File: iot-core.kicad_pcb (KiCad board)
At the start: 2 copper layers, 34 x 61.2 mm, 49 parts, among them P1 USB, P10 CONN_01X01, P11 CONN_01X01, P2 CONN_01X02, P3 CONN_01X16, P4 CONN_01X04, P5 CONN_01X16, P6 CONN_01X03, P7 CONN_01X03, P8 CONN_01X01, P9 CONN_01X01, SW1 SW1, SW2 SW_PUSH_SMALL_H, U1 LP2985LV, U2 STM32F103C8Tx, U3 ESP-07v2, Y1 8MHz

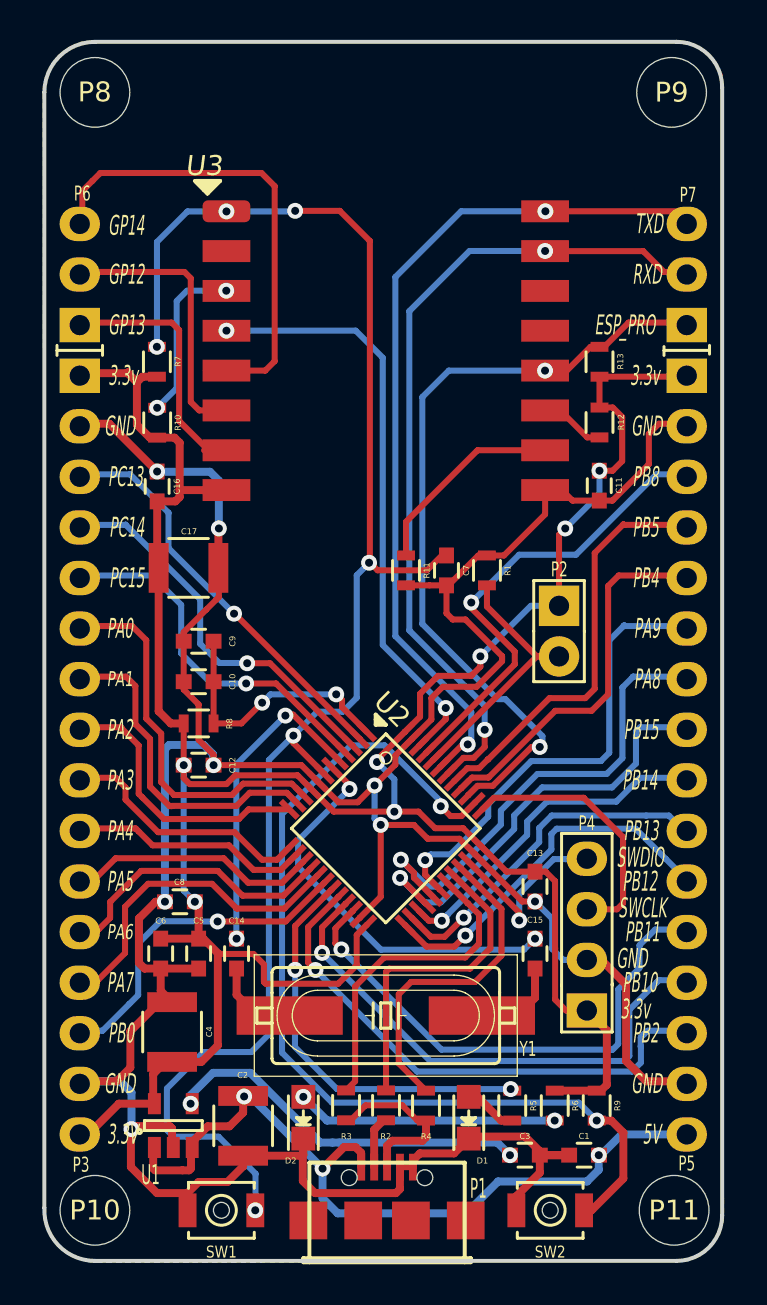
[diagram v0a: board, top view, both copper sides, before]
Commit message: Modified README file, rename project, add gerber file, anh 3d. ADD lib ESP8266 & BUTTON
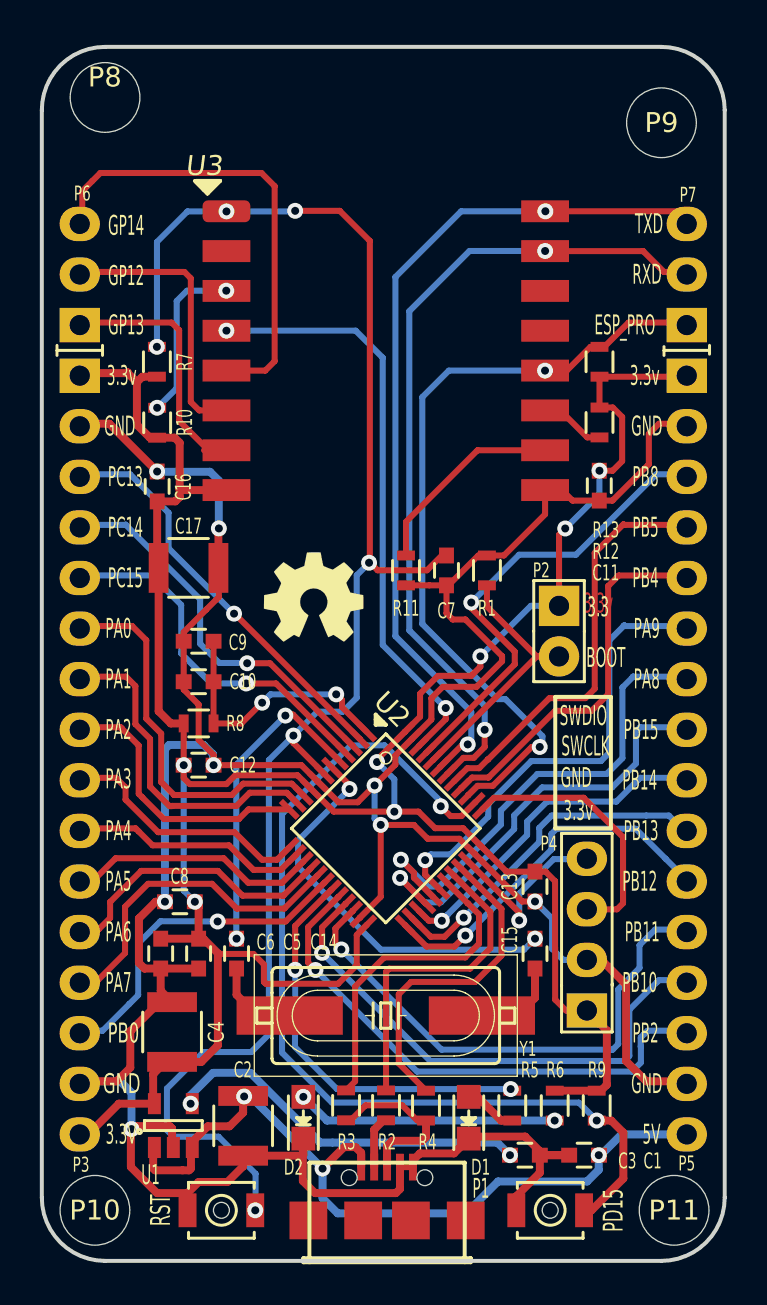
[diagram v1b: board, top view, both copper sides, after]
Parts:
- added G***: logo5_silkscreen-front_5mm, logo:logo5_silkscreen-front_5mm, F.Cu at (118.4, 102.6)
- SW1: value SW1 -> RST
- moved P9 1.61 mm to (135.9, 78.7)
- moved P8 0.57 mm to (108.0, 77.5)
- renumbered SW2 to PD15
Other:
- board size 34 x 61.2 mm -> 34.3 x 61 mm
- board text added: "3.3"
- board text added: "BOOT"
